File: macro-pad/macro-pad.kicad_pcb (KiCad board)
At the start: 2 copper layers, 31.5 x 55.5 mm, 4 parts, among them SW1 SW_Push, SW2 SW_Push, SW3 SW_Push, U1 MOUDLE-SEEEDUINO-XIAO

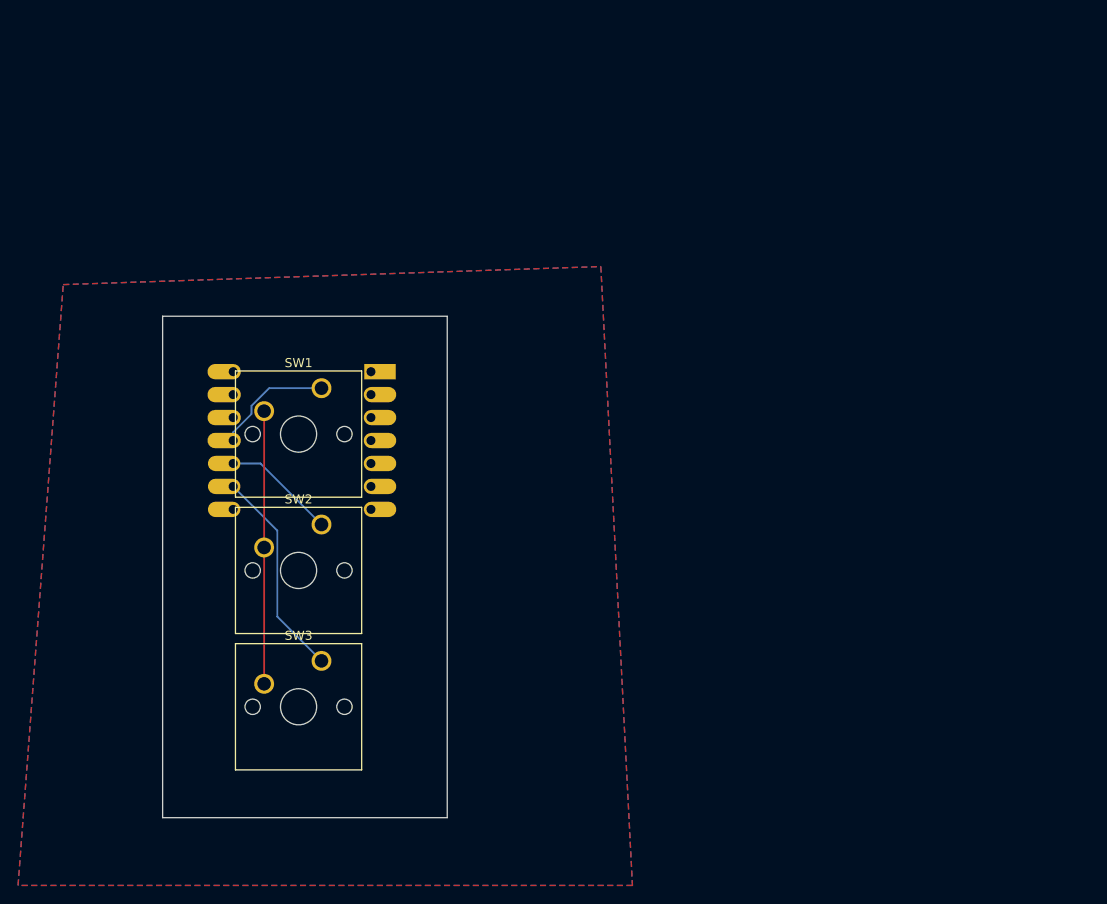
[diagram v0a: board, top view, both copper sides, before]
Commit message: added gerber files
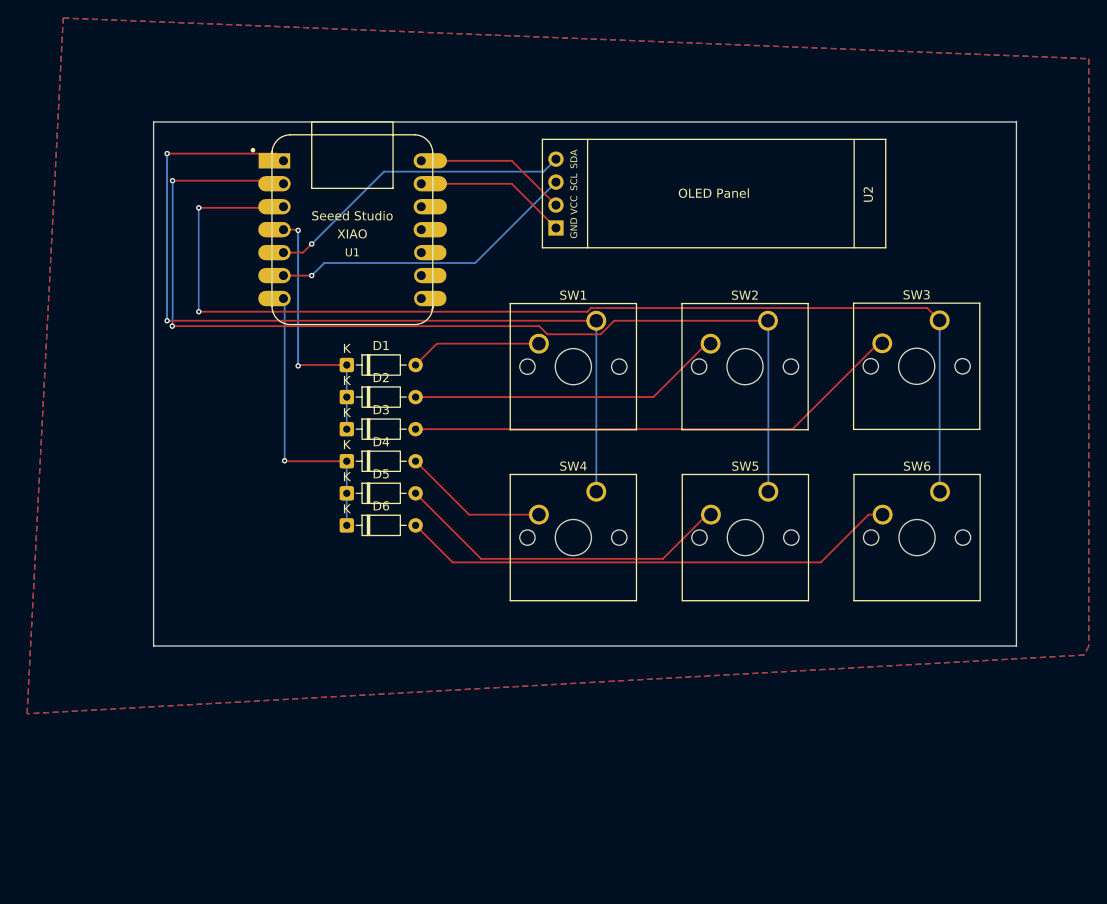
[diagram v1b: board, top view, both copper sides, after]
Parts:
- added D1: 1N4148, Diode_THT:D_DO-35_SOD27_P7.62mm_Horizontal, F.Cu at (157.4, 68.4)
- added D2: 1N4148, Diode_THT:D_DO-35_SOD27_P7.62mm_Horizontal, F.Cu at (157.4, 72.0)
- added D3: 1N4148, Diode_THT:D_DO-35_SOD27_P7.62mm_Horizontal, F.Cu at (157.4, 75.5)
- added D4: 1N4148, Diode_THT:D_DO-35_SOD27_P7.62mm_Horizontal, F.Cu at (157.4, 79.0)
- added D5: 1N4148, Diode_THT:D_DO-35_SOD27_P7.62mm_Horizontal, F.Cu at (157.4, 82.6)
- added D6: 1N4148, Diode_THT:D_DO-35_SOD27_P7.62mm_Horizontal, F.Cu at (157.4, 86.2)
- added SW4: SW_Push_45deg, Button_Switch_Keyboard:SW_Cherry_MX_1.00u_PCB, F.Cu at (185.0, 82.4)
- added SW5: SW_Push_45deg, Button_Switch_Keyboard:SW_Cherry_MX_1.00u_PCB, F.Cu at (204.0, 82.4)
- added SW6: SW_Push_45deg, Button_Switch_Keyboard:SW_Cherry_MX_1.00u_PCB, F.Cu at (223.0, 82.4)
- added U2: ER_OLEDM0.91_1x-I2C, KiCad-SSD1306-0.91-OLED-4pin-128x32:SSD1306-0.91-OLED-4pin-128x32, F.Cu at (217.0, 55.4)
- SW1, SW2, SW3: value SW_Push -> SW_Push_45deg
- U1: moved to F.Cu
- moved SW3 78.1 mm to (223.0, 63.5)
- moved SW2 54.3 mm to (204.0, 63.5)
- moved SW1 31.3 mm to (185.0, 63.5)
- moved U1 24.0 mm to (158.0, 53.4), turned to 0 degrees
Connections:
- SW1 pad 1: Net-(U1-PA6_A10_D10_MOSI) -> C0
- SW1 pad 2: GND -> Net-(D1-A)
- SW2 pad 1: Net-(U1-PA5_A9_D9_MISO) -> C1
- SW2 pad 2: GND -> Net-(D2-A)
- SW3 pad 1: Net-(U1-PA7_A8_D8_SCK) -> C2
- SW3 pad 2: GND -> Net-(D3-A)
- U1 pad 1: unconnected-(U1-PA02_A0_D0-Pad1) -> C0
- U1 pad 10: Net-(U1-PA5_A9_D9_MISO) -> unconnected-(U1-PA5_A9_D9_MISO-Pad10)
- U1 pad 11: Net-(U1-PA6_A10_D10_MOSI) -> unconnected-(U1-PA6_A10_D10_MOSI-Pad11)
- U1 pad 14: unconnected-(U1-5V-Pad14) -> INP
- U1 pad 2: unconnected-(U1-PA4_A1_D1-Pad2) -> C1
- U1 pad 3: unconnected-(U1-PA10_A2_D2-Pad3) -> C2
- U1 pad 4: unconnected-(U1-PA11_A3_D3-Pad4) -> R0
- U1 pad 5: unconnected-(U1-PA8_A4_D4_SDA-Pad5) -> SDA
- U1 pad 6: unconnected-(U1-PA9_A5_D5_SCL-Pad6) -> SCL
- U1 pad 7: unconnected-(U1-PB08_A6_D6_TX-Pad7) -> R1
- U1 pad 9: Net-(U1-PA7_A8_D8_SCK) -> unconnected-(U1-PA7_A8_D8_SCK-Pad9)
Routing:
- net C2: track 0.00 -> 122.6 mm, vias 0 -> 2
- net C1: track 0.00 -> 114.4 mm, vias 0 -> 2
- net C0: track 0.00 -> 98.1 mm, vias 0 -> 2
- net Net-(D3-A): track 0.00 -> 55.6 mm
- net Net-(D6-A): track 0.00 -> 55.6 mm
- net Net-(D5-A): track 0.00 -> 37.7 mm
- net Net-(D2-A): track 0.00 -> 35.1 mm
- net SCL: track 0.00 -> 34.4 mm, vias 0 -> 1
- net SDA: track 0.00 -> 34.4 mm, vias 0 -> 1
- net R1: track 0.00 -> 32.0 mm, vias 0 -> 1
- net R0: track 0.00 -> 29.2 mm, vias 0 -> 2
- net Net-(U1-PA7_A8_D8_SCK): track 23.4 -> 0.00 mm
- net INP: track 0.00 -> 16.9 mm
- net Net-(D4-A): track 0.00 -> 16.1 mm
- net Net-(D1-A): track 0.00 -> 14.6 mm
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- added copper zone on B.Cu, net (none)
- added copper zone on F.Cu, net (none)
- removed copper zone on B.Cu, net Net-(U1-PA6_A10_D10_MOSI)
- removed copper zone on F.Cu, net Net-(U1-PA6_A10_D10_MOSI)
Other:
- board size 31.5 x 55.5 mm -> 95.5 x 58 mm
